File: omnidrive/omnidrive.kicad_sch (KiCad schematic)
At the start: 43 parts, among them J1 AudioJack3, J2 Conn_01x01_Pin, J3 Conn_01x01_Pin, SW1 SW_SPDT, SW2 SW_SPDT, SW3 SW_SPST, SW4 SW_SPDT, U1 TL072, U2 TL072

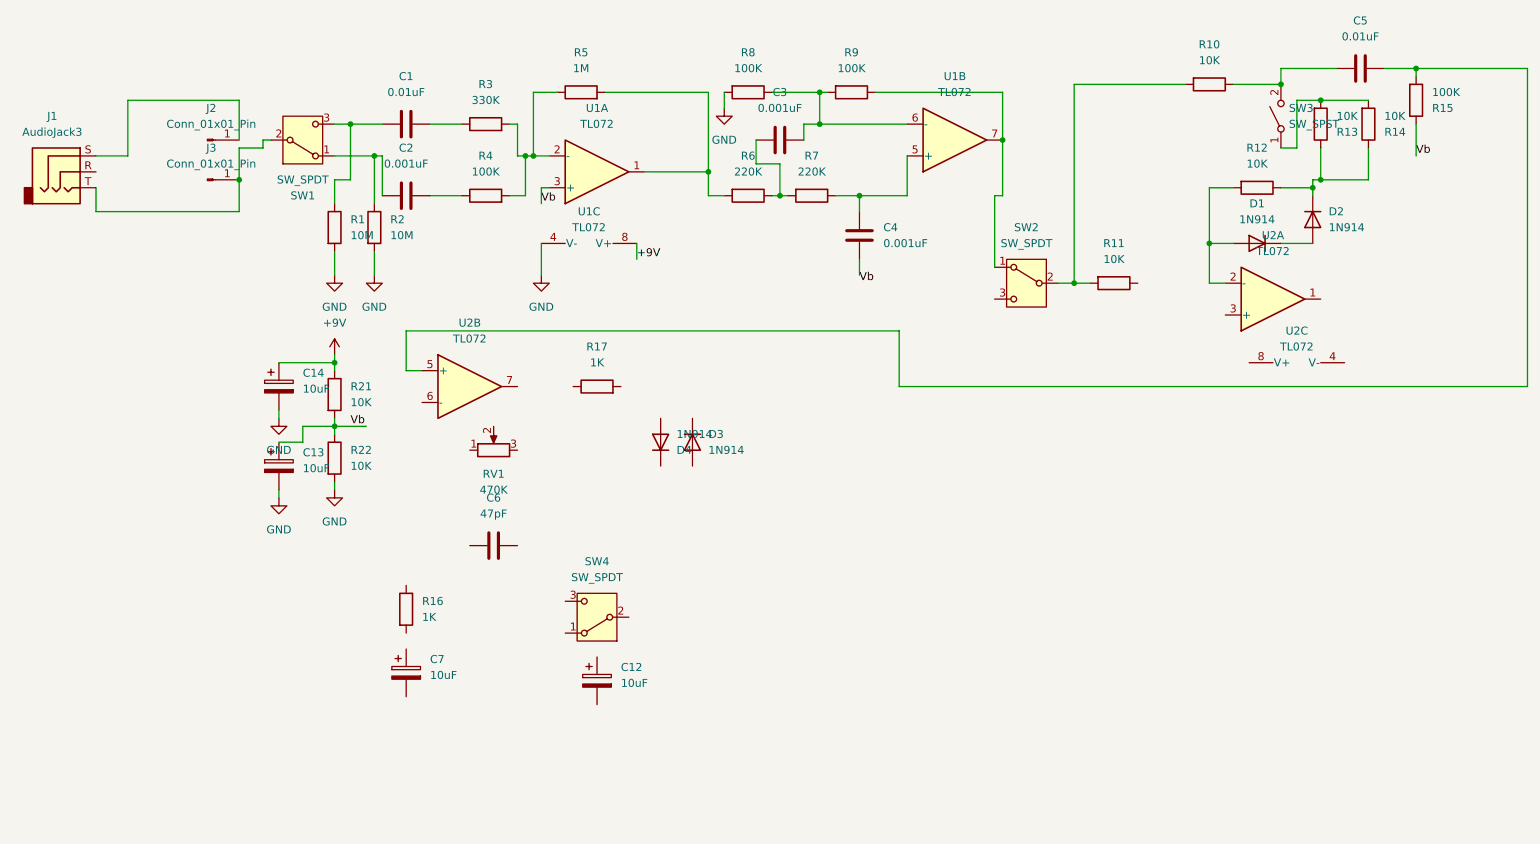
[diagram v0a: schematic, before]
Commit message: annotation and ERC check
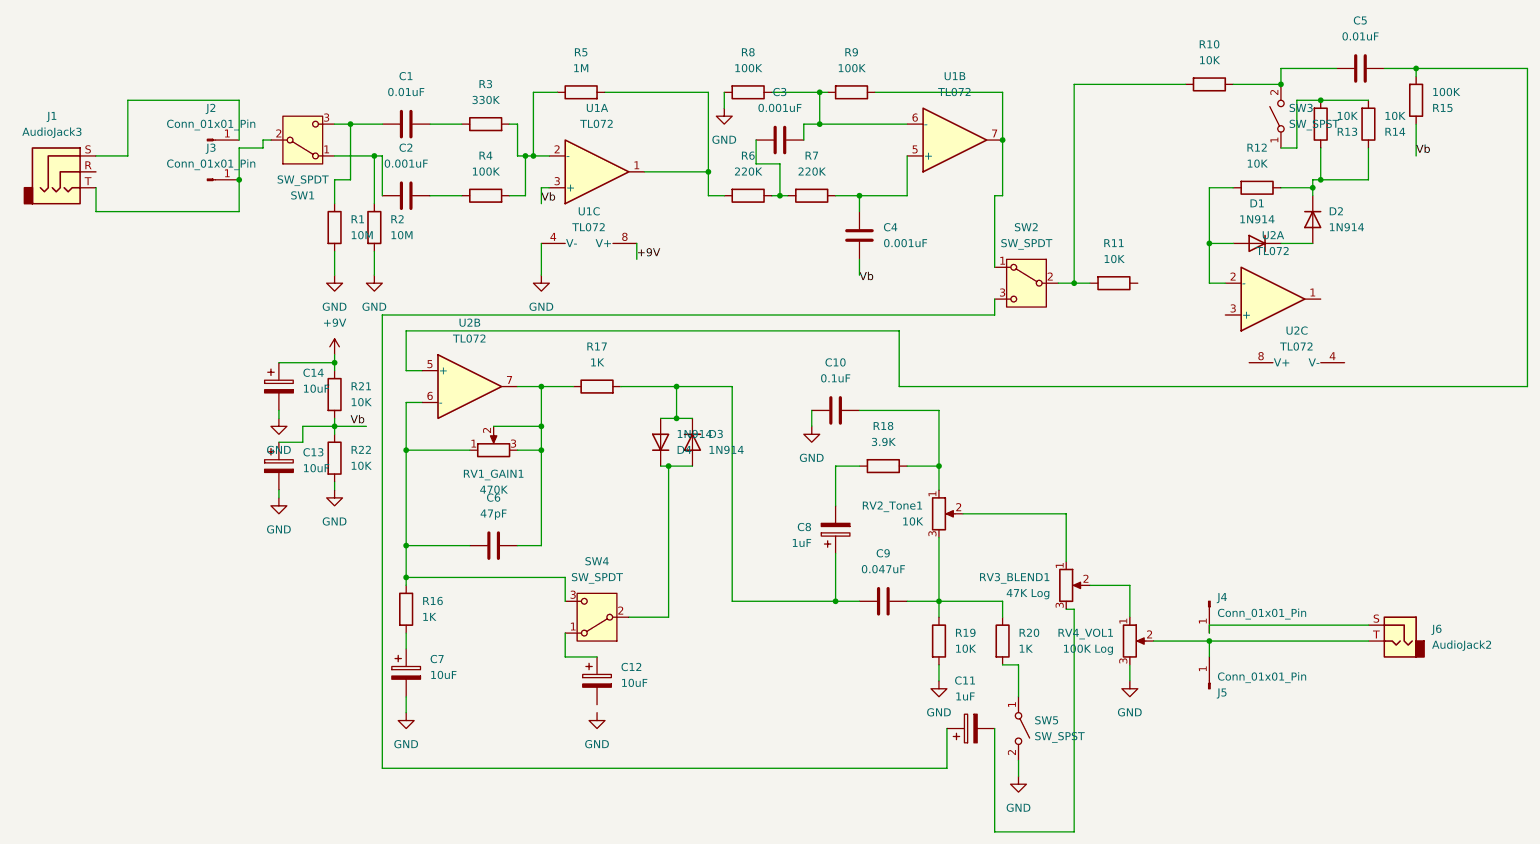
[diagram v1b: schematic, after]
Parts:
- added C10: 0.1uF, symbol Device:C
- added C11, C8: 1uF, symbol Device:C_Polarized
- added C9: 0.047uF, symbol Device:C
- added J4, J5: Conn_01x01_Pin, symbol Connector:Conn_01x01_Pin
- added J6: AudioJack2, symbol Connector_Audio:AudioJack2
- added R18: 3.9K, symbol Device:R
- added R19: 10K, symbol Device:R
- added R20: 1K, symbol Device:R
- added RV2_Tone1: 10K, symbol Device:R_Potentiometer
- added RV3_BLEND1: 47K Log, symbol Device:R_Potentiometer
- added RV4_VOL1: 100K Log, symbol Device:R_Potentiometer
- added SW5: SW_SPST, symbol Switch:SW_SPST
- renumbered RV1 to RV1_GAIN1
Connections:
- net GND: now also C7.2, C10.1, R19.2, RV4_VOL1.3, SW5.2 (B)
- net at R17.1: now also C6.2, RV1_GAIN1.2, RV1_GAIN1.3, U2.7
- net at R17.2: now also D3.1 (K), D4.2 (A), C8.1, C9.1
- net at D4.1 (K): now also D3.2 (A), SW4.2 (B)
- net at SW4.1 (A): now also C12.1
- net at SW4.3 (C): now also C6.1, R16.1, RV1_GAIN1.1, U2.6 (-)
- net at R16.2: now also C7.1
- net at SW2.3 (C): now also C11.1
- new net: C11.2, RV3_BLEND1.3
- new net: C8.2, R18.2
- new net: C9.2, R19.1, R20.1, RV2_Tone1.3
- new net: C10.2, R18.1, RV2_Tone1.1
- new net: RV3_BLEND1.2, RV4_VOL1.1
- new net: J5.1 (Pin_1), J6.T, RV4_VOL1.2
- new net: R20.2, SW5.1 (A)
- new net: RV2_Tone1.2, RV3_BLEND1.1
- new net: J4.1 (Pin_1), J6.S
